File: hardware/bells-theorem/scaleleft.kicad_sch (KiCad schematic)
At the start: 16 parts, among them U12 MCP6004

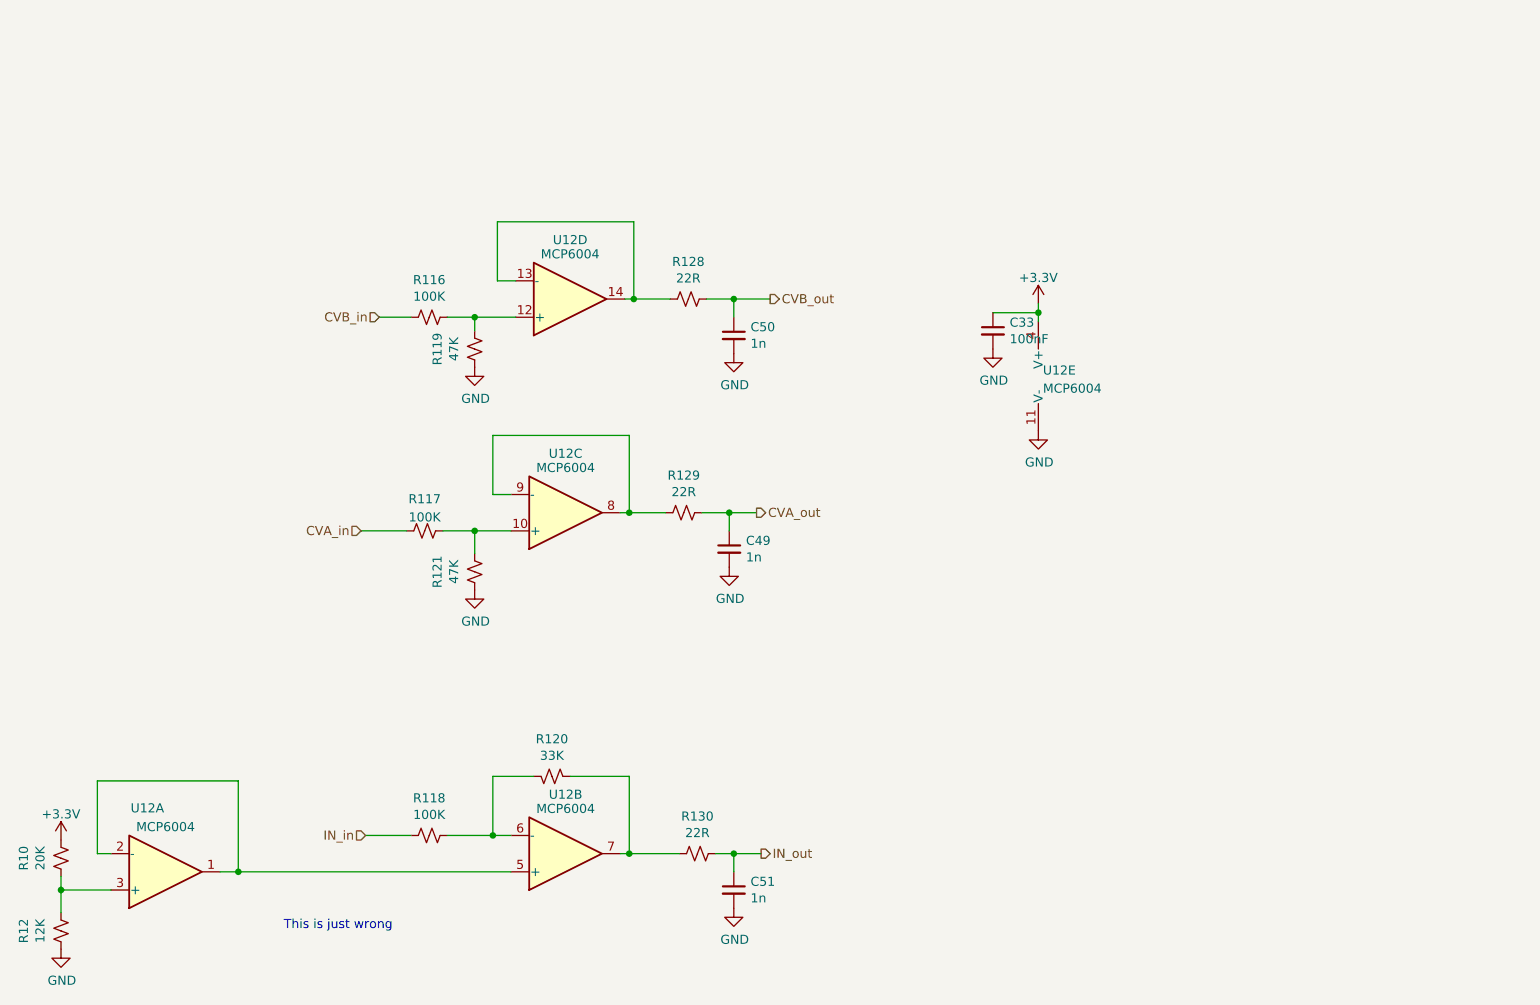
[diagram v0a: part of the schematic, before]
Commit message: checking in old outstanding changes prior to debugging with Claude Code
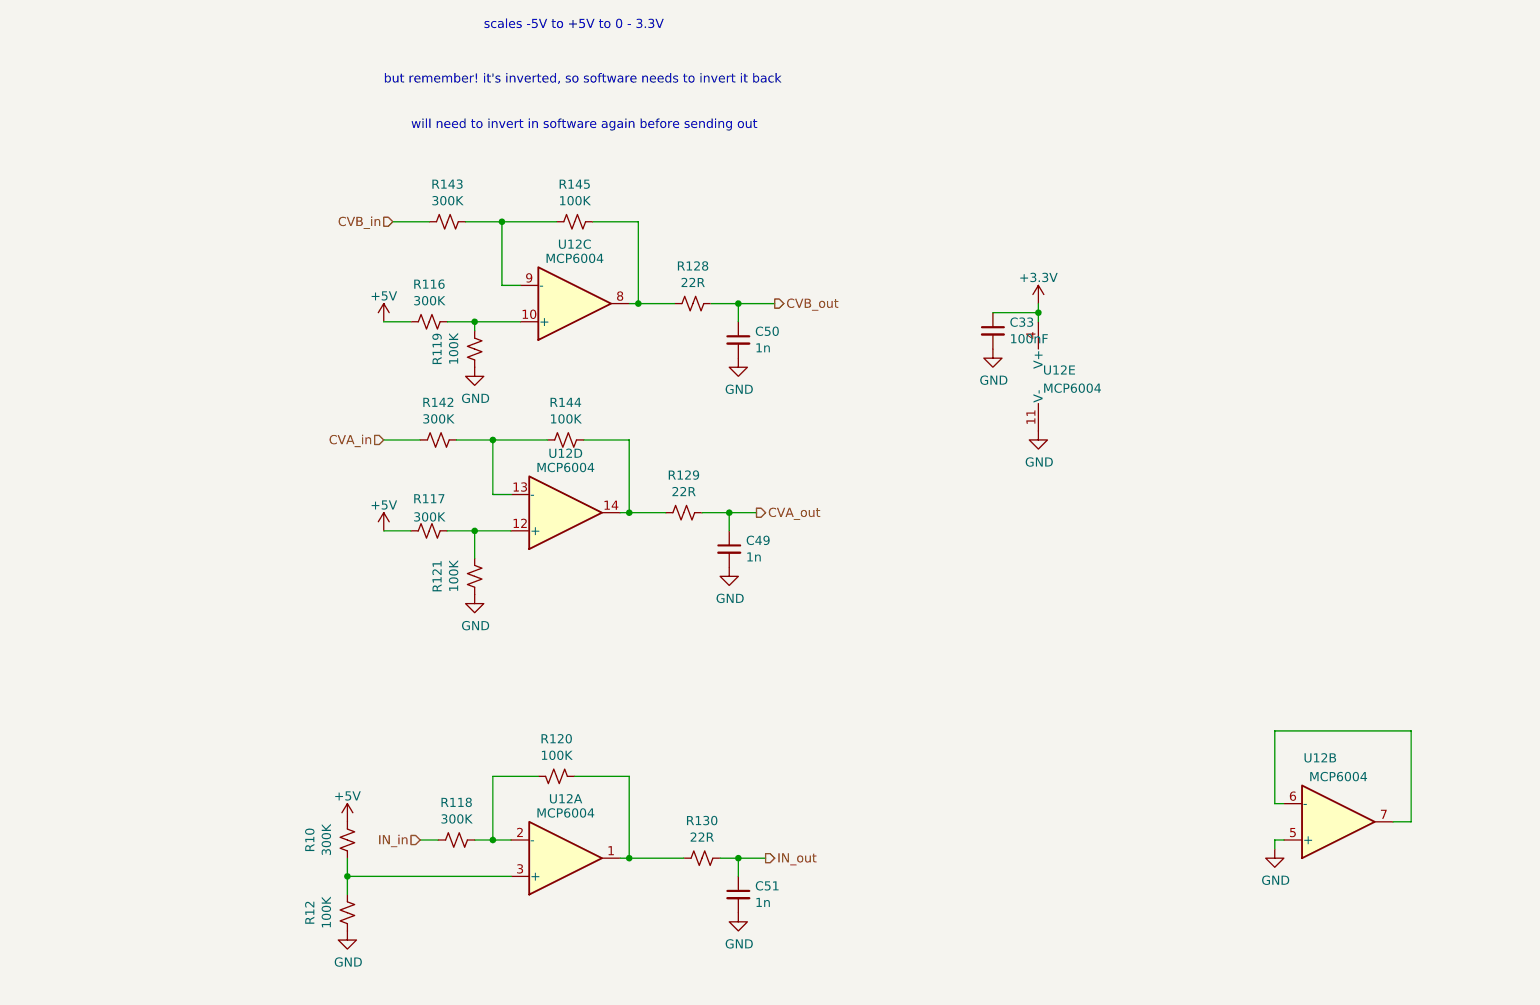
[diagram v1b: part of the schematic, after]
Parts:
- added R142, R143: 300K, Resistor_SMD:R_0805_2012Metric_Pad1.20x1.40mm_HandSolder, symbol Device:R_Small_US
- added R144, R145: 100K, Resistor_SMD:R_0805_2012Metric_Pad1.20x1.40mm_HandSolder, symbol Device:R_Small_US
- R10: value 20K -> 300K
- R116, R117, R118: value 100K -> 300K
- R119, R121: value 47K -> 100K
- R12: value 12K -> 100K
- R120: value 33K -> 100K
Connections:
- net +3V3: no longer R10.1
- net CVA_in: now also R142.2; no longer R117.2
- net CVB_in: now also R143.2; no longer R116.2
- net GND: now also U12.5 (+)
- net at R116.1, R119.1: now also U12.10 (+); no longer U12.12 (+)
- net at R117.1, R121.1: now also U12.12 (+); no longer U12.10 (+)
- net at R118.1, R120.1: now also U12.2 (-); no longer U12.6 (-)
- net at R120.2, R130.2: now also U12.1; no longer U12.7
- net at R10.2, R12.1: now also U12.3 (+); no longer U12.3 (+)
- new net: R129.2, R144.1, U12.14
- new net: R128.2, R145.1, U12.8
- new net: U12.6 (-), U12.7
- new net: R143.1, R145.2, U12.9 (-)
- new net: R142.1, R144.2, U12.13 (-)
- new net +5V: R10.1, R116.2, R117.2
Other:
- note added: "but remember! it's inverted, so software needs to invert it back"
- note added: "scales -5V to +5V to 0 - 3.3V"
- note added: "will need to invert in software again before sending out"
- note removed: "This is just wrong"
- moved on the sheet: C50, C51, R10, R116, R117, R118, R12, R120, R121, R128, R130, U12A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
